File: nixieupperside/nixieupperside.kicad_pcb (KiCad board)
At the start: 2 copper layers, 6 parts, among them J1 Conn_01x04, J2 Conn_01x10

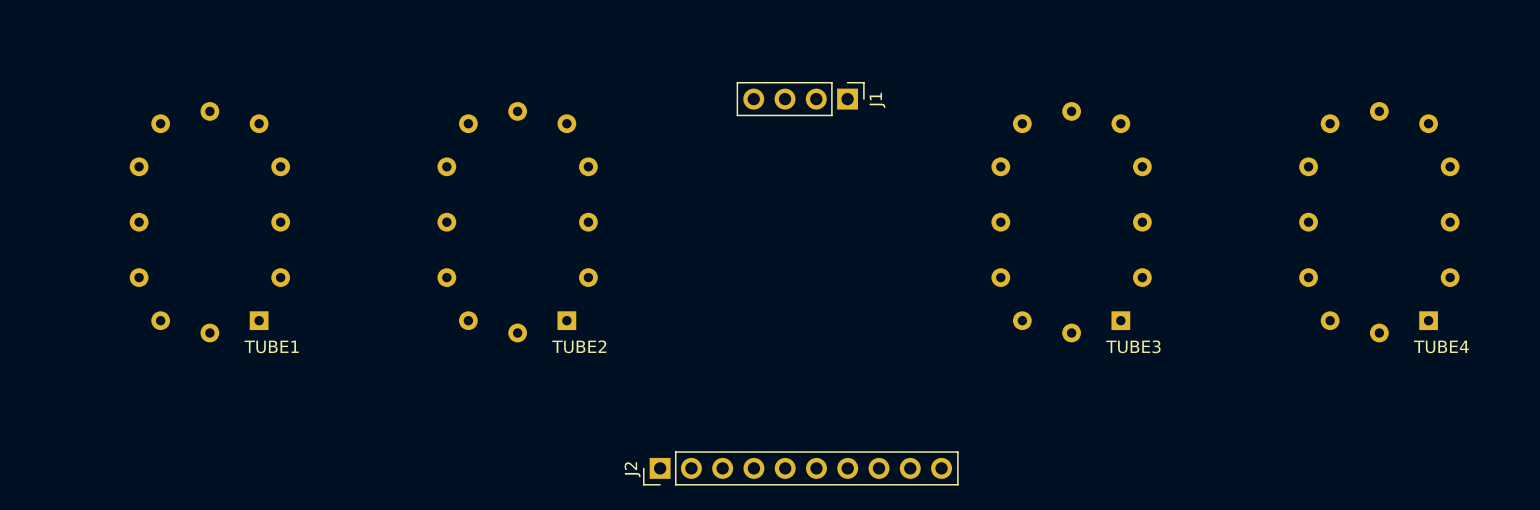
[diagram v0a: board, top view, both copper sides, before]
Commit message: accomplished
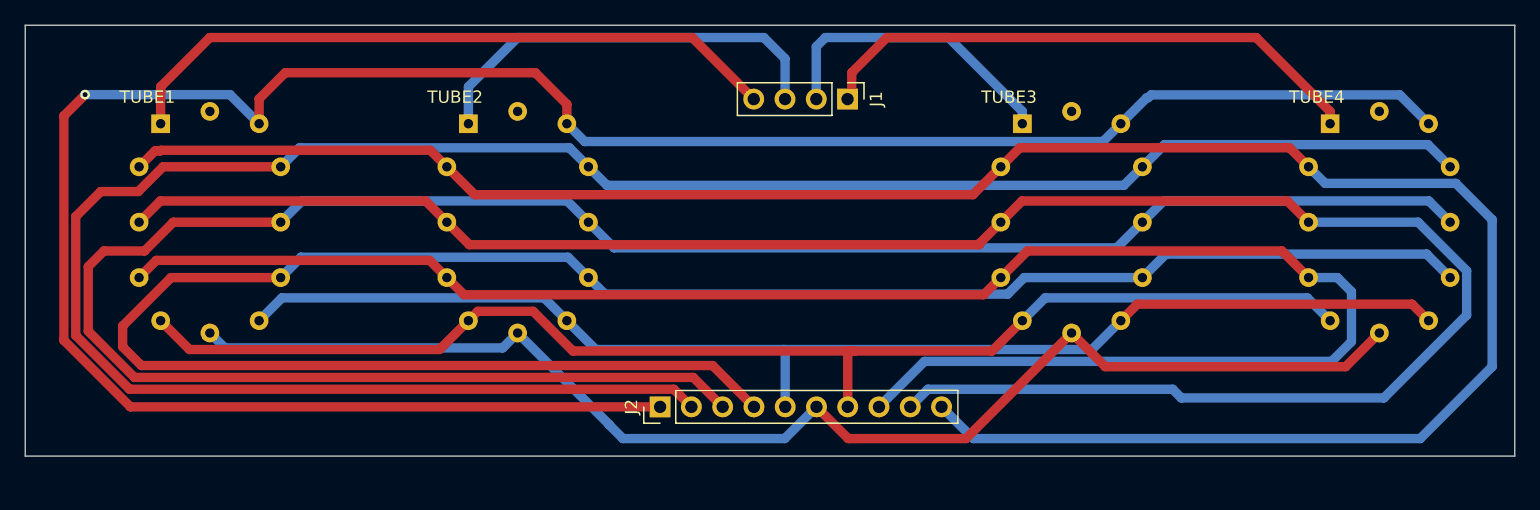
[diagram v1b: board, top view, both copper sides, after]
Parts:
- moved J2 5.00 mm to (101.6, 50.0)
- turned TUBE1 to 180 degrees
- turned TUBE2 to 180 degrees
- turned TUBE3 to 180 degrees
- turned TUBE4 to 180 degrees
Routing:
- net 1: track 0.00 -> 190.1 mm, vias 0 -> 1
- net 2: track 0.00 -> 179.4 mm
- net 0: track 0.00 -> 176.1 mm
- net 3: track 0.00 -> 176.0 mm
- net 4: track 0.00 -> 168.5 mm
- net 9: track 0.00 -> 166.4 mm
- net 8: track 0.00 -> 147.7 mm
- net 6: track 0.00 -> 107.5 mm
- net 7: track 0.00 -> 106.2 mm
- net 5: track 0.00 -> 104.3 mm
- net ANODE_1: track 0.00 -> 54.9 mm
- net ANODE_4: track 0.00 -> 45.8 mm
- net ANODE_2: track 0.00 -> 34.4 mm
- net ANODE_3: track 0.00 -> 24.8 mm
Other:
- board outline added: 121 x 35 mm
